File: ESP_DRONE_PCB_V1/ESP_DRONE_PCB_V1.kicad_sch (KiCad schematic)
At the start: 38 parts, among them J1 6130XX11121_61300811121, J2 6130XX11121_61300811121, Q1 SI2300DS-T1-GE3, Q2 SI2300DS-T1-GE3, Q3 SI2300DS-T1-GE3, Q4 SI2300DS-T1-GE3, U1 MPU-6050

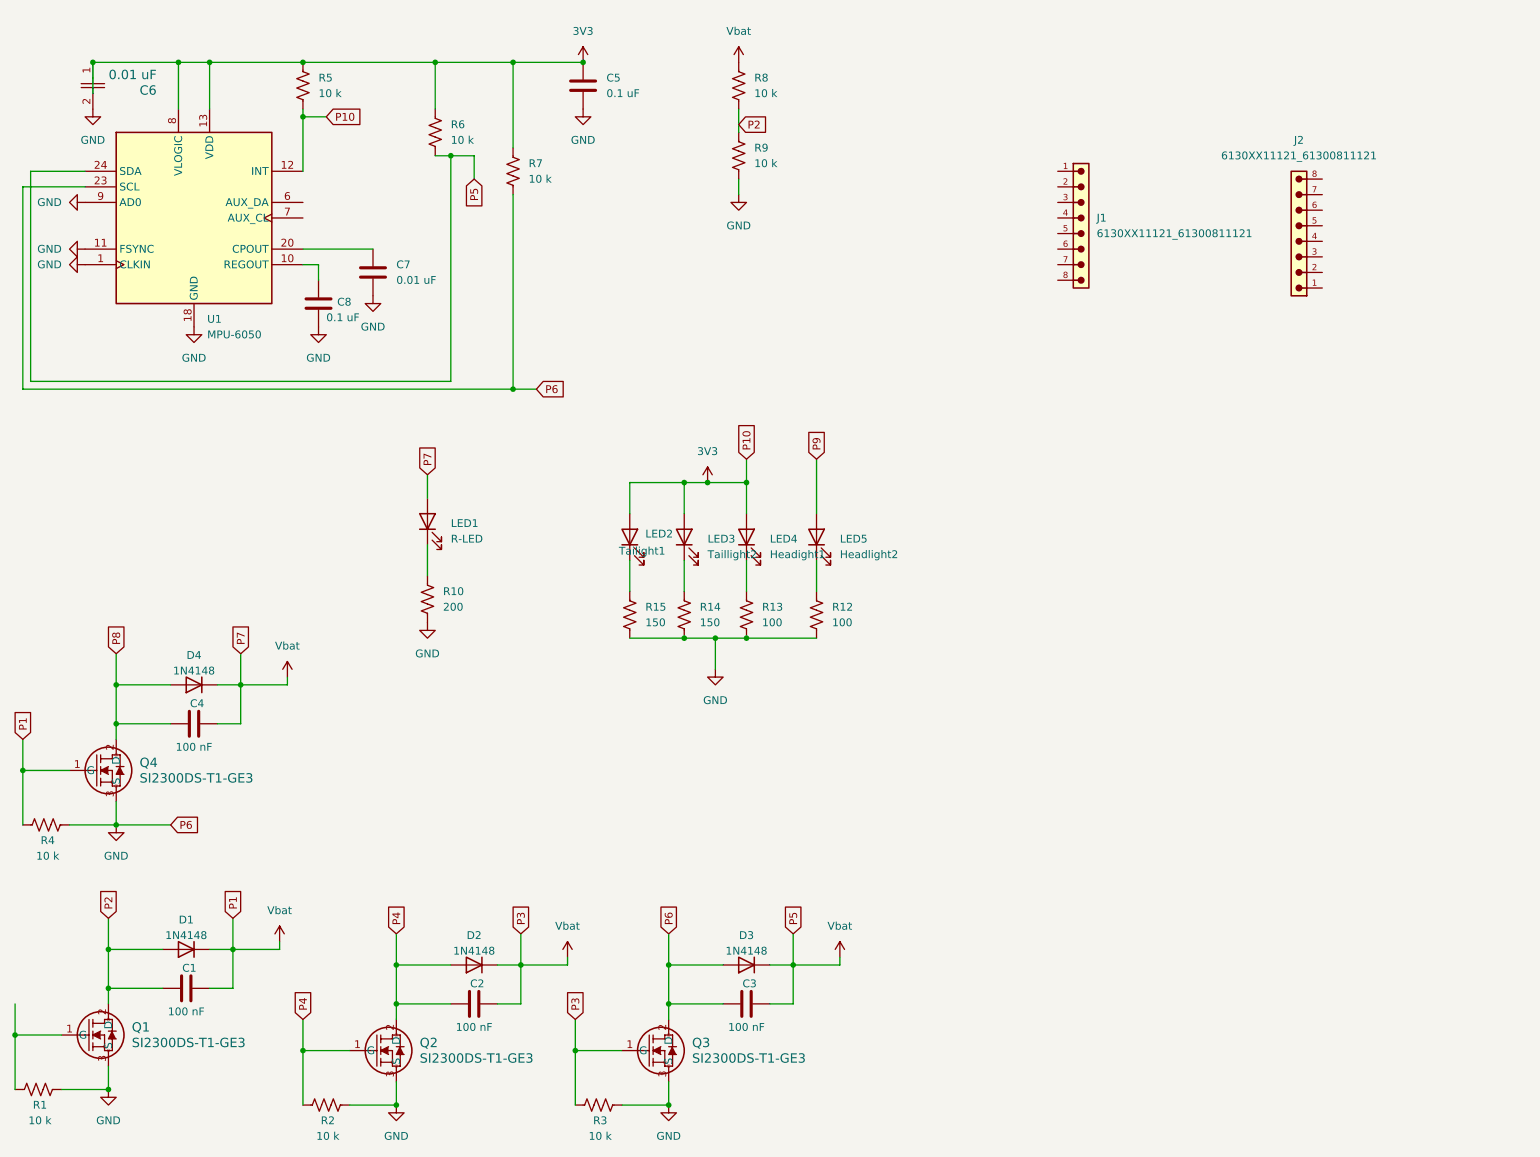
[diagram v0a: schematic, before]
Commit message: Add files via upload
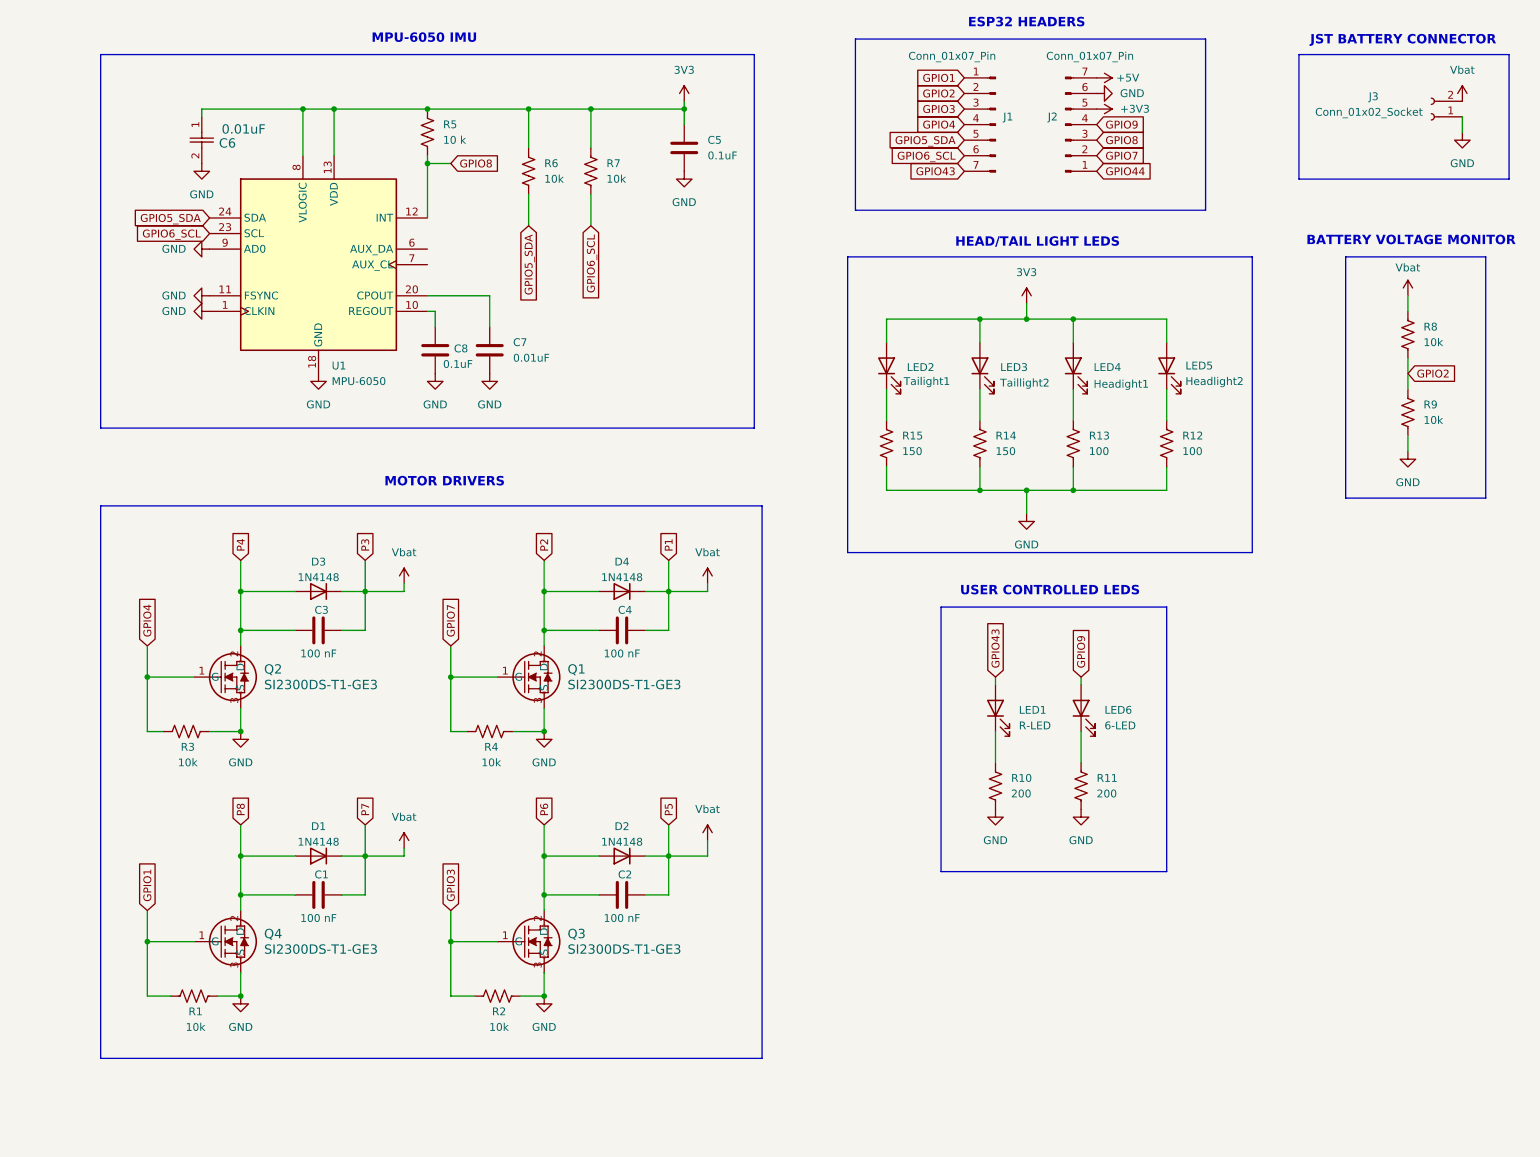
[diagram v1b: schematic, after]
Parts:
- removed J1, J2: 6130XX11121_61300811121, 6130XX11121_61300811121:61300811121, symbol 3rdParty_Symbols:6130XX11121_61300811121
- added J1, J2: Conn_01x07_Pin, symbol Connector:Conn_01x07_Pin
- added J3: Conn_01x02_Socket, symbol Connector:Conn_01x02_Socket
- added LED6: 6-LED, symbol Device:LED
- added R11: 200, symbol Device:R_US
- C5, C8: value 0.1 uF -> 0.1uF
- C6, C7: value 0.01 uF -> 0.01uF
- R1, R2, R3, R4, R6, R7, R8, R9: value 10 k -> 10k
- renumbered Q4 to Q1, Q3 to Q2, Q2 to Q3, Q1 to Q4
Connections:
- net P9 is gone; now on net 3V3: LED5.2 (A)
- net 3V3: no longer R5.2, U1.12 (INT)
- net GND: now also J2.6 (Pin_6), J3.1 (Pin_1), R11.2; no longer C3.1, D3.2 (A), Q2.2 (D), R7.2, U1.23 (SCL)
- net P2: now also C4.1, D4.2 (A), Q1.2 (D); no longer C1.1, D1.2 (A), Q4.2 (D), R8.2, R9.1
- net P4: now also C3.1, D3.2 (A), Q2.2 (D); no longer C2.1, D2.2 (A), Q3.1 (G), Q3.2 (D), R2.1
- net P8: now also C1.1, D1.2 (A), Q4.2 (D); no longer C4.1, D4.2 (A), Q1.2 (D)
- net Vbat: now also J3.2 (Pin_2); no longer LED1.2 (A), Q1.1 (G), Q2.1 (G), R3.1, R4.1, R6.2, U1.24 (SDA)
- net GPIO1: now reaches Q4.1 (G), R1.1
- net GPIO1: now also J1.1 (Pin_1)
- new net: LED6.1 (K), R11.1
- new net +3V3: J2.5 (Pin_5)
- new net +5V: J2.7 (Pin_7)
- new net GPIO2: J1.2 (Pin_2), R8.2, R9.1
- new net GPIO3: J1.3 (Pin_3), Q3.1 (G), R2.1
- new net GPIO4: J1.4 (Pin_4), Q2.1 (G), R3.1
- new net GPIO43: J1.7 (Pin_7), LED1.2 (A)
- new net GPIO44: J2.1 (Pin_1)
- new net GPIO5_SDA: J1.5 (Pin_5), R6.2, U1.24 (SDA)
- new net GPIO6_SCL: J1.6 (Pin_6), R7.2, U1.23 (SCL)
- new net GPIO7: J2.2 (Pin_2), Q1.1 (G), R4.1
- new net GPIO8: J2.3 (Pin_3), R5.2, U1.12 (INT)
- new net GPIO9: J2.4 (Pin_4), LED6.2 (A)
- new net P6: C2.1, D2.2 (A), Q3.2 (D)
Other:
- note added: "BATTERY VOLTAGE MONITOR"
- note added: "ESP32 HEADERS"
- note added: "HEAD/TAIL LIGHT LEDS"
- note added: "JST BATTERY CONNECTOR"
- note added: "MOTOR DRIVERS"
- note added: "MPU-6050 IMU"
- note added: "USER CONTROLLED LEDS"
- moved on the sheet: C1, C2, C3, C4, C5, C6, C7, C8, D1, D2, D3, D4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
